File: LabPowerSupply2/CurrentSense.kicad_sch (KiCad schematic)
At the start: 10 parts

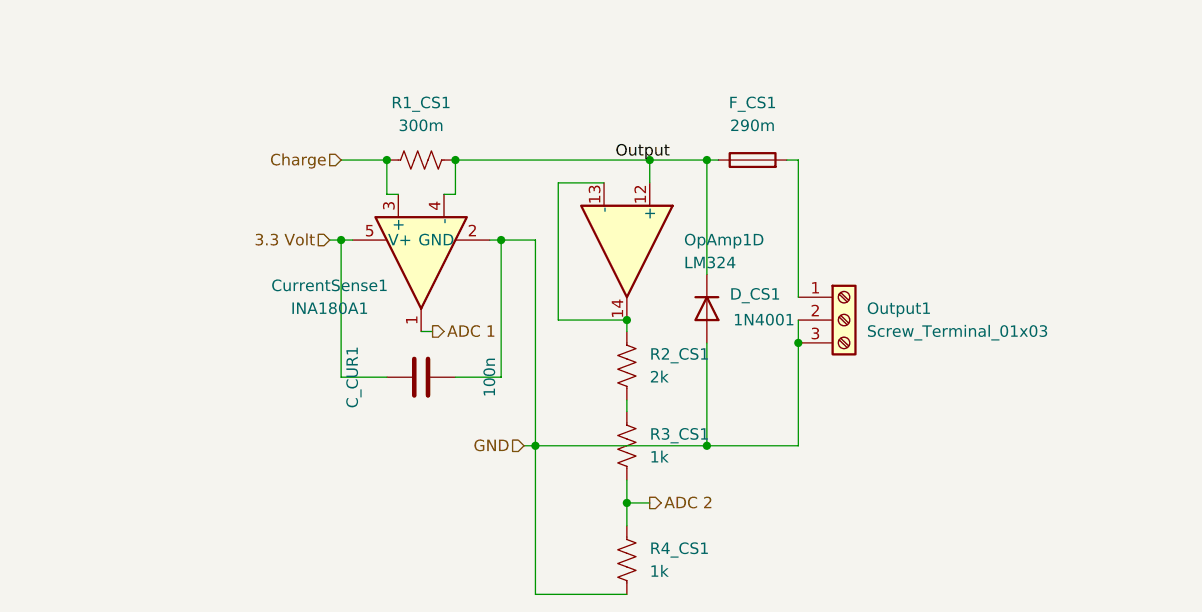
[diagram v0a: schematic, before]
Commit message: Beautifing the Schematic
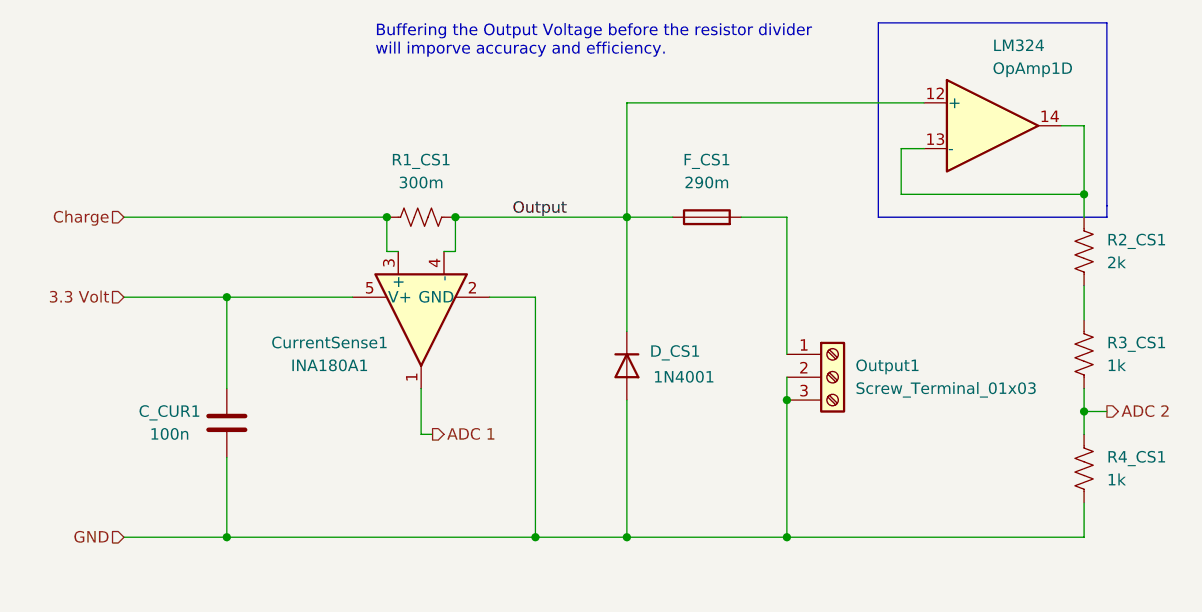
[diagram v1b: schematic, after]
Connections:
- net 3.3 Volt: now also C_CUR1.1; no longer C_CUR1.2
- net ADC 2: now also R3_CS1.1, R4_CS1.2; no longer R3_CS1.2, R4_CS1.1
- net GND: now also C_CUR1.2, R4_CS1.1; no longer C_CUR1.1, R4_CS1.2
- net at OpAmp1.13 (-), OpAmp1.14: now also R2_CS1.2; no longer R2_CS1.1
- new net: R2_CS1.1, R3_CS1.2
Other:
- note added: "Buffering the Output Voltage before the resistor divider will imporve accuracy and efficiency."
- moved on the sheet: C_CUR1, CurrentSense1, D_CS1, F_CS1, OpAmp1D, Output1, R1_CS1, R2_CS1, R3_CS1, R4_CS1
